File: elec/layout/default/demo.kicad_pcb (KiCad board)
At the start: 4 copper layers, 25 x 25 mm, 34 parts, among them U1 ?, U2 ?, U3 ?, U4 ?, U5 ?, U6 KMR211NGLFS (Tactile Switches), U7 ?, U8 ?

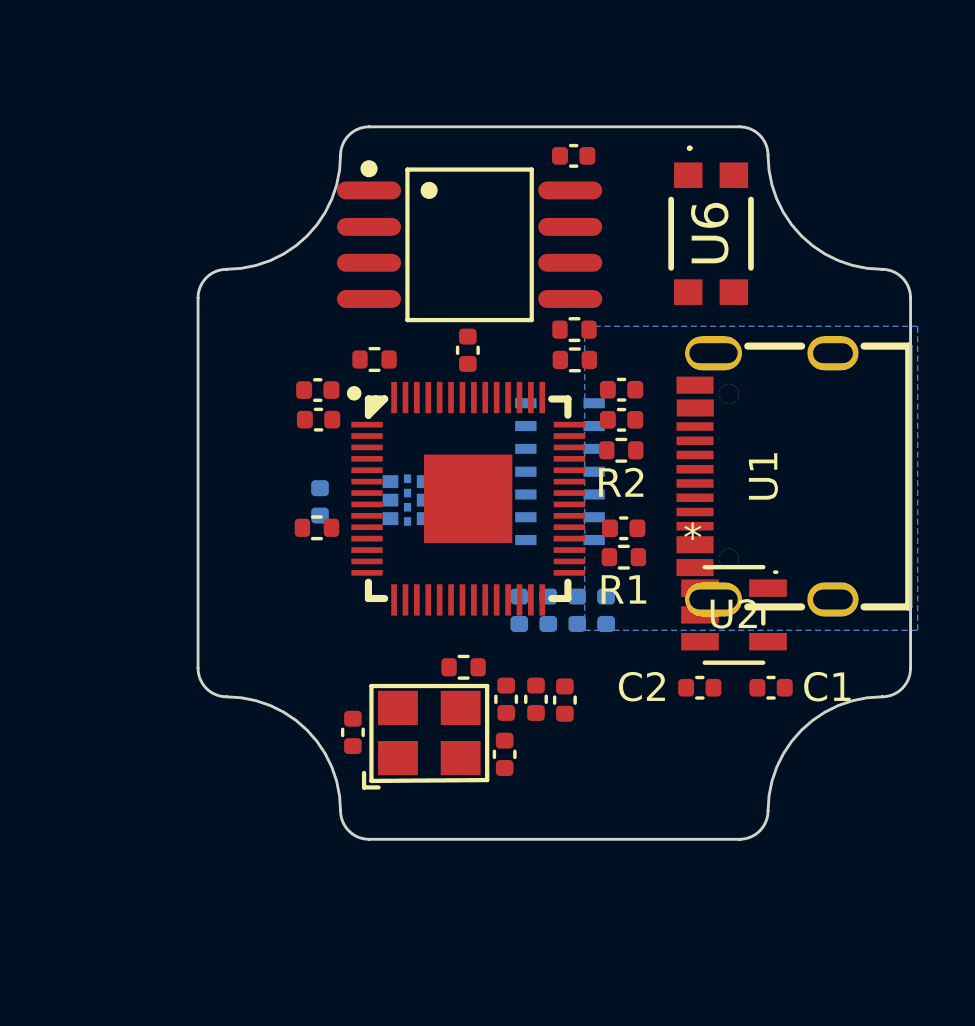
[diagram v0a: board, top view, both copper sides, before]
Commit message: [DEMO] better
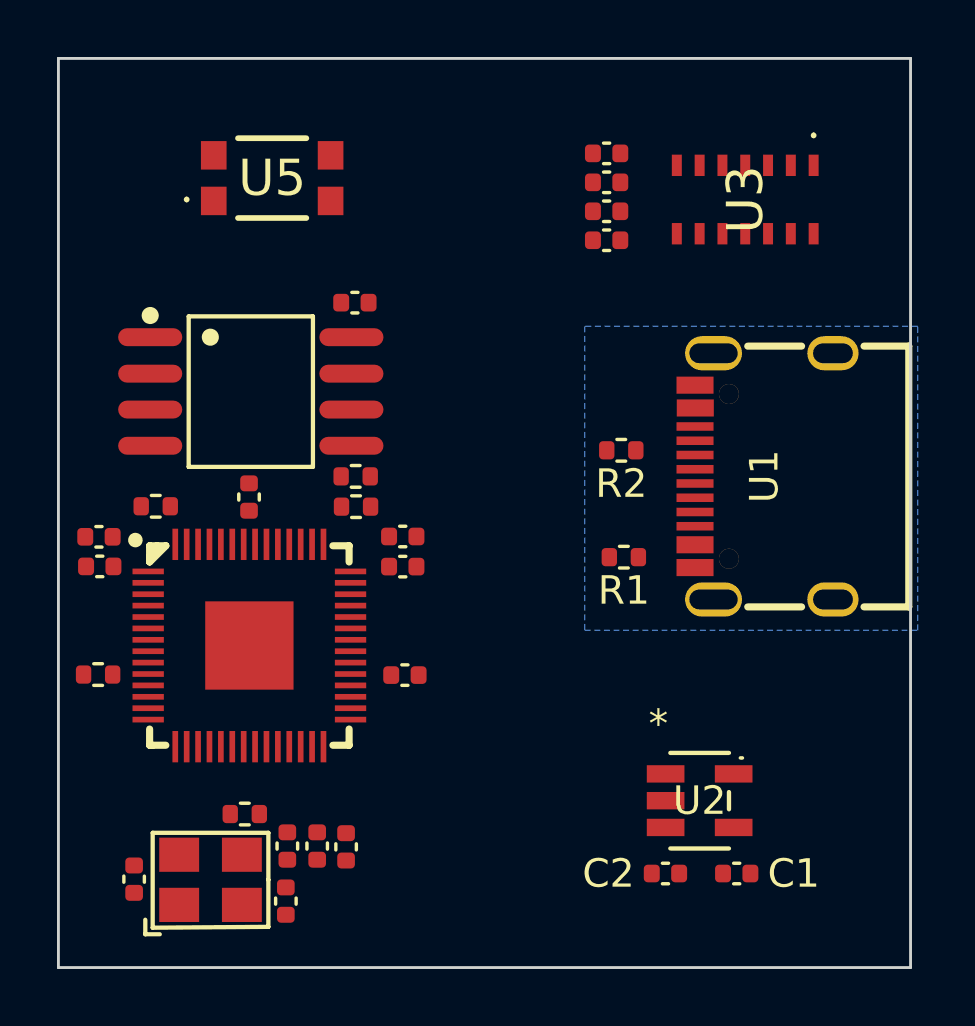
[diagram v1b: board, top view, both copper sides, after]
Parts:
- removed the C7 at (134.3, 103.2)
- removed the U4 at (137.3, 103.1)
- C3, C4, C5, C6, U3: moved to F.Cu
- R1, R2: value 62.5mW Thick Film Resistors 50V ±100ppm/℃ ±1% 5.1kΩ 0402 Chip Resistor - Surface Mount ROHS -> 62.5mW Thick Film Resistors 50V ±100ppm/℃ ±1% 4.7kΩ 0402 Chip Resistor - Surface Mount ROHS
- moved C3 16.0 mm to (144.3, 90.9), turned to 180 degrees
- moved U5 15.5 mm to (132.6, 91.8), turned to 180 degrees
- moved C4 15.1 mm to (144.3, 91.9), turned to 180 degrees
- moved C5 14.1 mm to (144.3, 93.0), turned to 180 degrees
- moved C6 13.3 mm to (144.3, 94.0), turned to 180 degrees
- moved U3 11.6 mm to (149.2, 92.6), turned to -90 degrees
- moved C13 9.24 mm to (137.3, 109.2)
- moved C14 9.24 mm to (135.5, 96.2)
- moved C7 9.24 mm to (127.8, 116.4)
- moved C8 9.24 mm to (133.1, 117.2)
- moved R4 9.24 mm to (128.5, 103.3)
- moved U7 9.24 mm to (131.9, 99.3)
- moved C11 9.24 mm to (126.5, 104.4)
- moved R5 9.24 mm to (131.6, 114.1)
- moved R6 9.24 mm to (135.5, 102.3)
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- renumbered C11 to C10, C12 to C11, C13 to C12, C14 to C13, C15 to C14, C16 to C15, C17 to C16, C18 to C17, C19 to C18, C8 to C7, C9 to C8, C10 to C9, U5 to U4, U6 to U5, U7 to U6, U8 to U7
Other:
- board size 25 x 25 mm -> 29.9 x 31.9 mm
